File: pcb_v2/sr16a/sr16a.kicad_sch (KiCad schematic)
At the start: 35 parts, among them J1 Conn_02x22_Top_Bottom, U1 74LS193, U2 74LS193, U3 74LS193, U4 74LS193, U5 74LS244, U6 74LS244, U7 74LS244, U8 74LS244, U9 74LS32

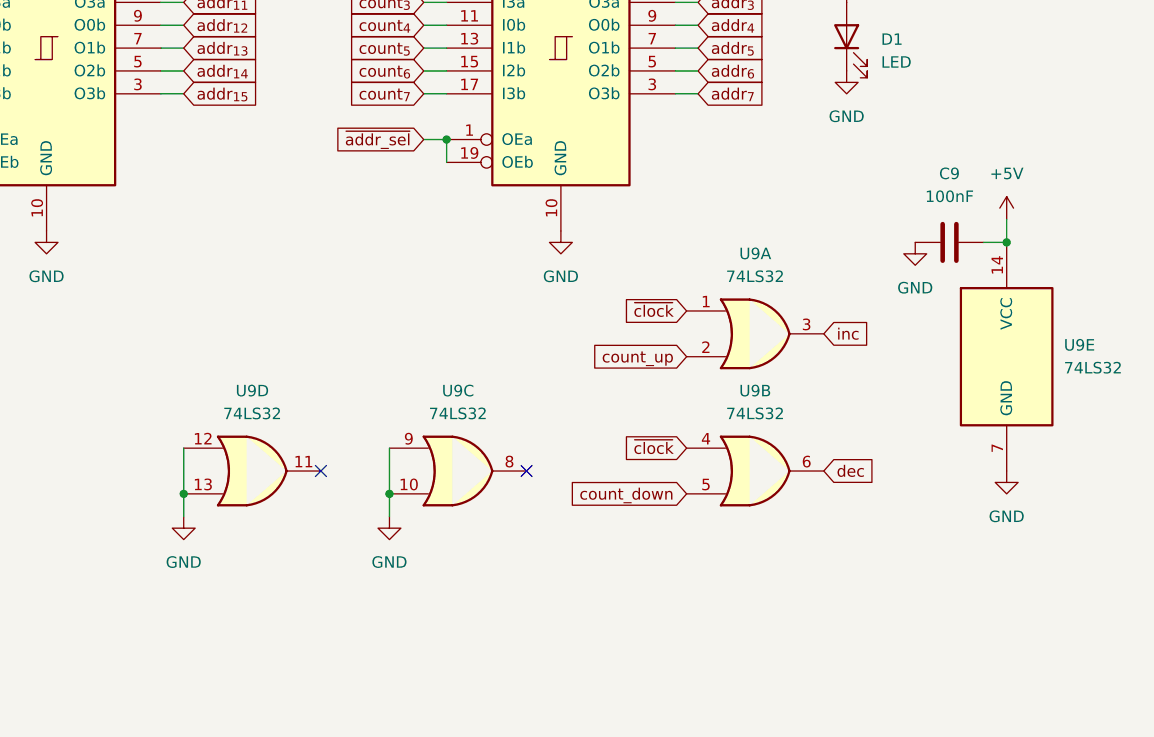
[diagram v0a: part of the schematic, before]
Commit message: arquivos do gdrive
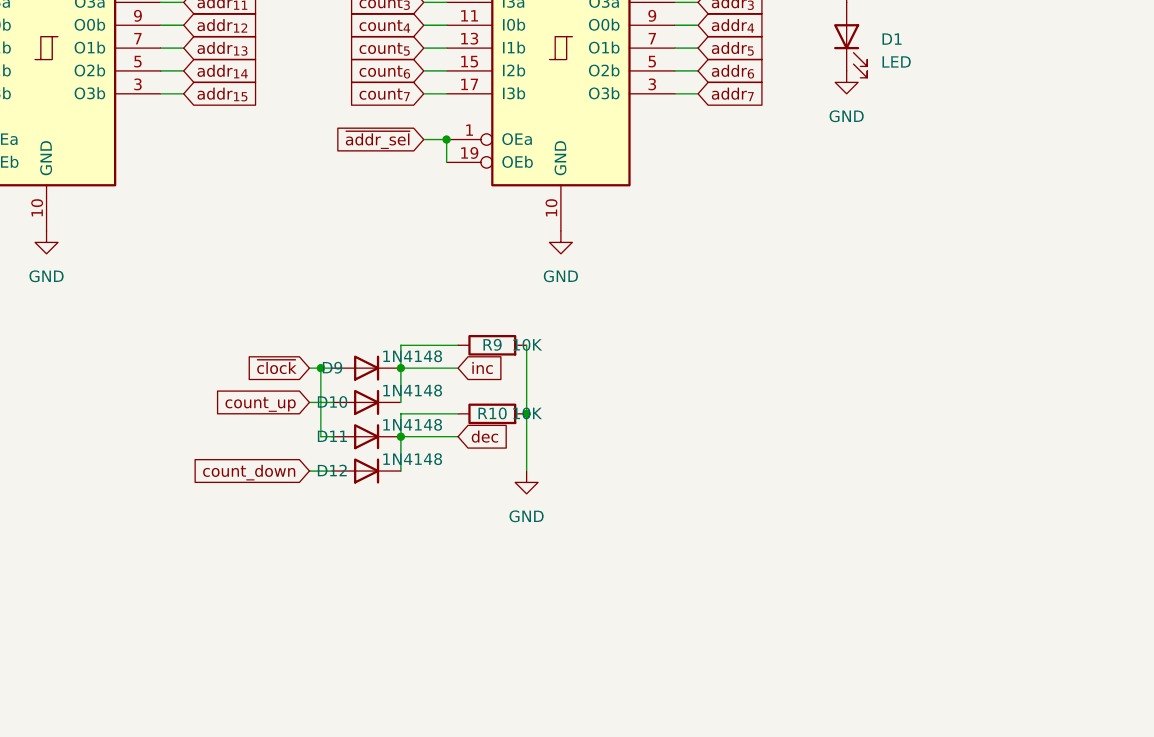
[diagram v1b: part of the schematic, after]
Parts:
- removed C9: 100nF, Capacitor_THT:C_Disc_D5.1mm_W3.2mm_P5.00mm, symbol Device:C
- removed U9: 74LS32, Package_DIP:DIP-14_W7.62mm, symbol 74xx:74LS32
- added D10, D11, D12, D9: 1N4148, Diode_THT:D_DO-35_SOD27_P7.62mm_Horizontal, symbol Diode:1N4148
- added R10, R9: 10K, Resistor_THT:R_Axial_DIN0207_L6.3mm_D2.5mm_P7.62mm_Horizontal, symbol Device:R
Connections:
- net GND: now also R10.2, R9.2
- net count_down: now also D12.2 (A)
- net count_up: now also D10.2 (A)
- net dec: now also D11.1 (K), D12.1 (K), R10.1
- net inc: now also D10.1 (K), D9.1 (K), R9.1
- net ~{clock}: now also D11.2 (A), D9.2 (A)
- no-connect marks 12 -> 10
